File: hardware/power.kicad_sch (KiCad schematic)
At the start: 20 parts, among them Q2 SI2347DS-T1-GE3, U7 NCP565D2T33R4G, U8 RSH3-2405S_H2

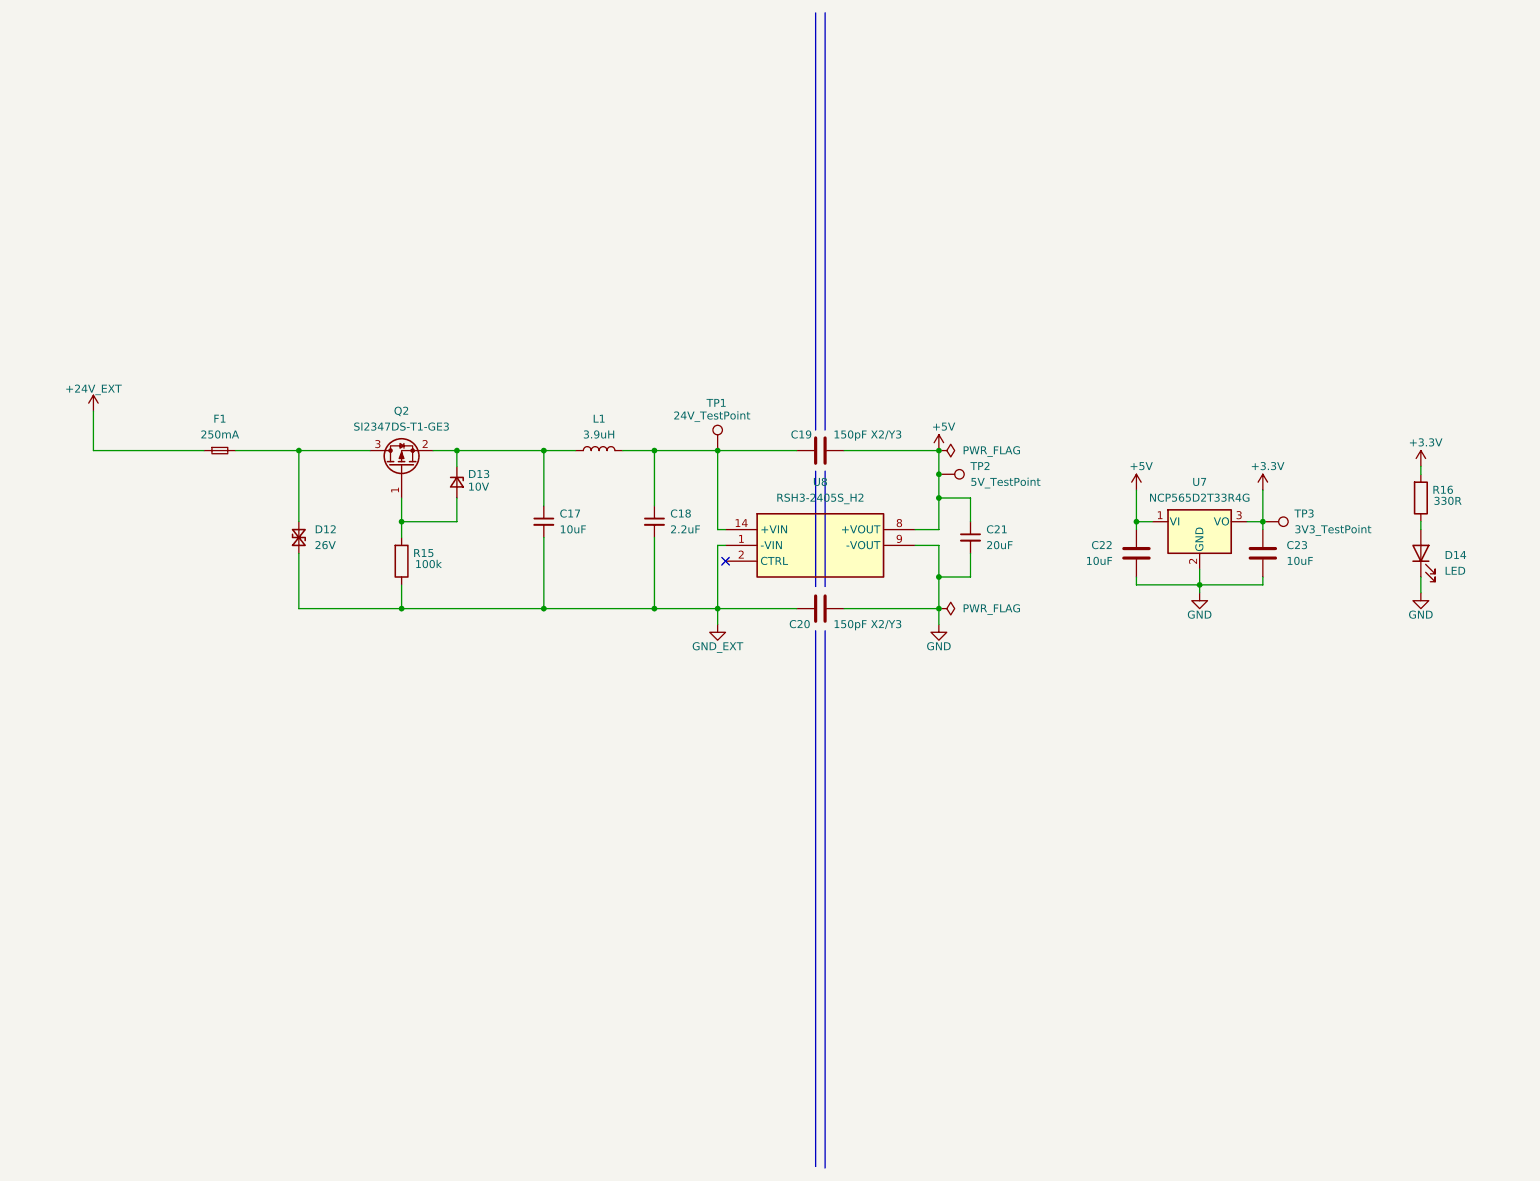
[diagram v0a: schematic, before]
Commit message: Some smaller fixes and final aesthetic changes
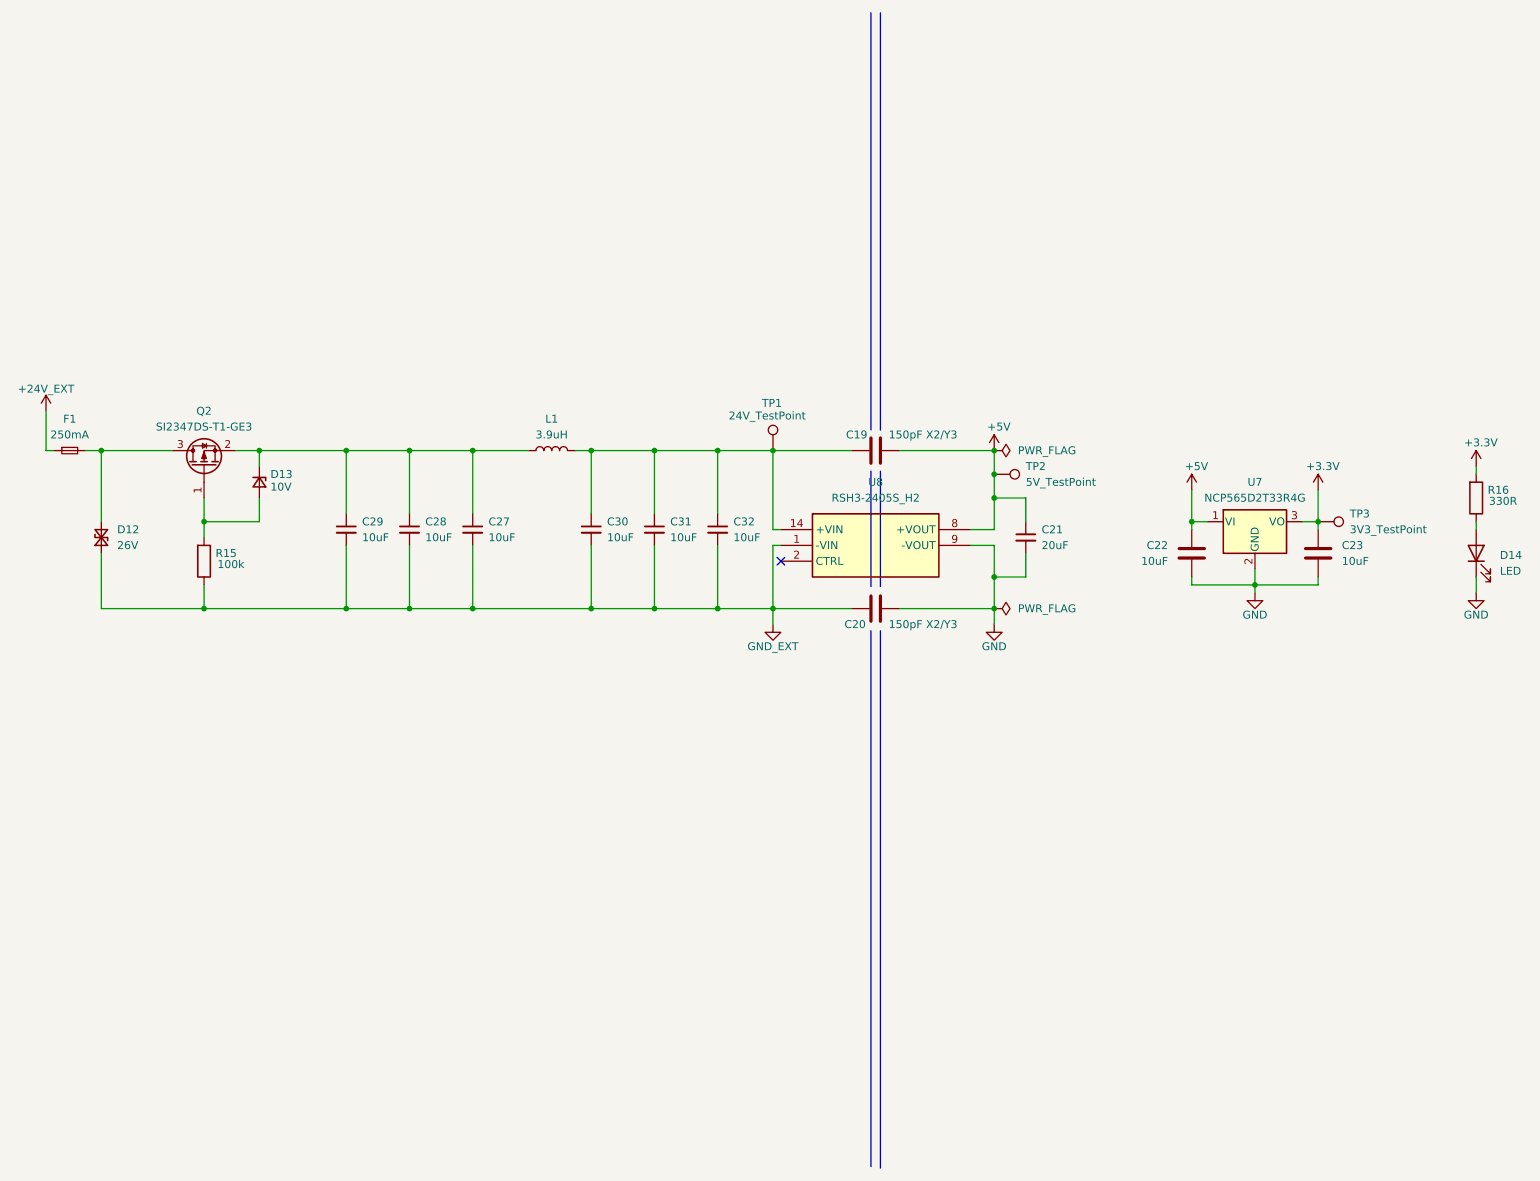
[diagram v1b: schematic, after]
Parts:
- removed C17: 10uF, 10uF24Vcap:CAPC6050X550N, symbol Device:C_Small
- removed C18: 2.2uF, Capacitor_SMD:C_1206_3216Metric_Pad1.33x1.80mm_HandSolder, symbol Device:C_Small
- added C27, C28, C29, C30, C31, C32: 10uF, Capacitor_SMD:C_1206_3216Metric, symbol Device:C_Small
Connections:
- net GND_EXT: now also C27.2, C28.2, C29.2, C30.2, C31.2, C32.2
- net at D13.1 (K), L1.1, Q2.2 (S): now also C27.1, C28.1, C29.1
- net at C19.1, L1.2, TP1.1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: now also C30.1, C31.1, C32.1
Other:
- company: Author: -> Author: Kacper Pawlak
- moved on the sheet: C19, C20, C21, C22, C23, D12, D13, D14, F1, L1, Q2, R15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
